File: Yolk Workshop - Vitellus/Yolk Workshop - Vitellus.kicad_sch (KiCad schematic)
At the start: 3 parts

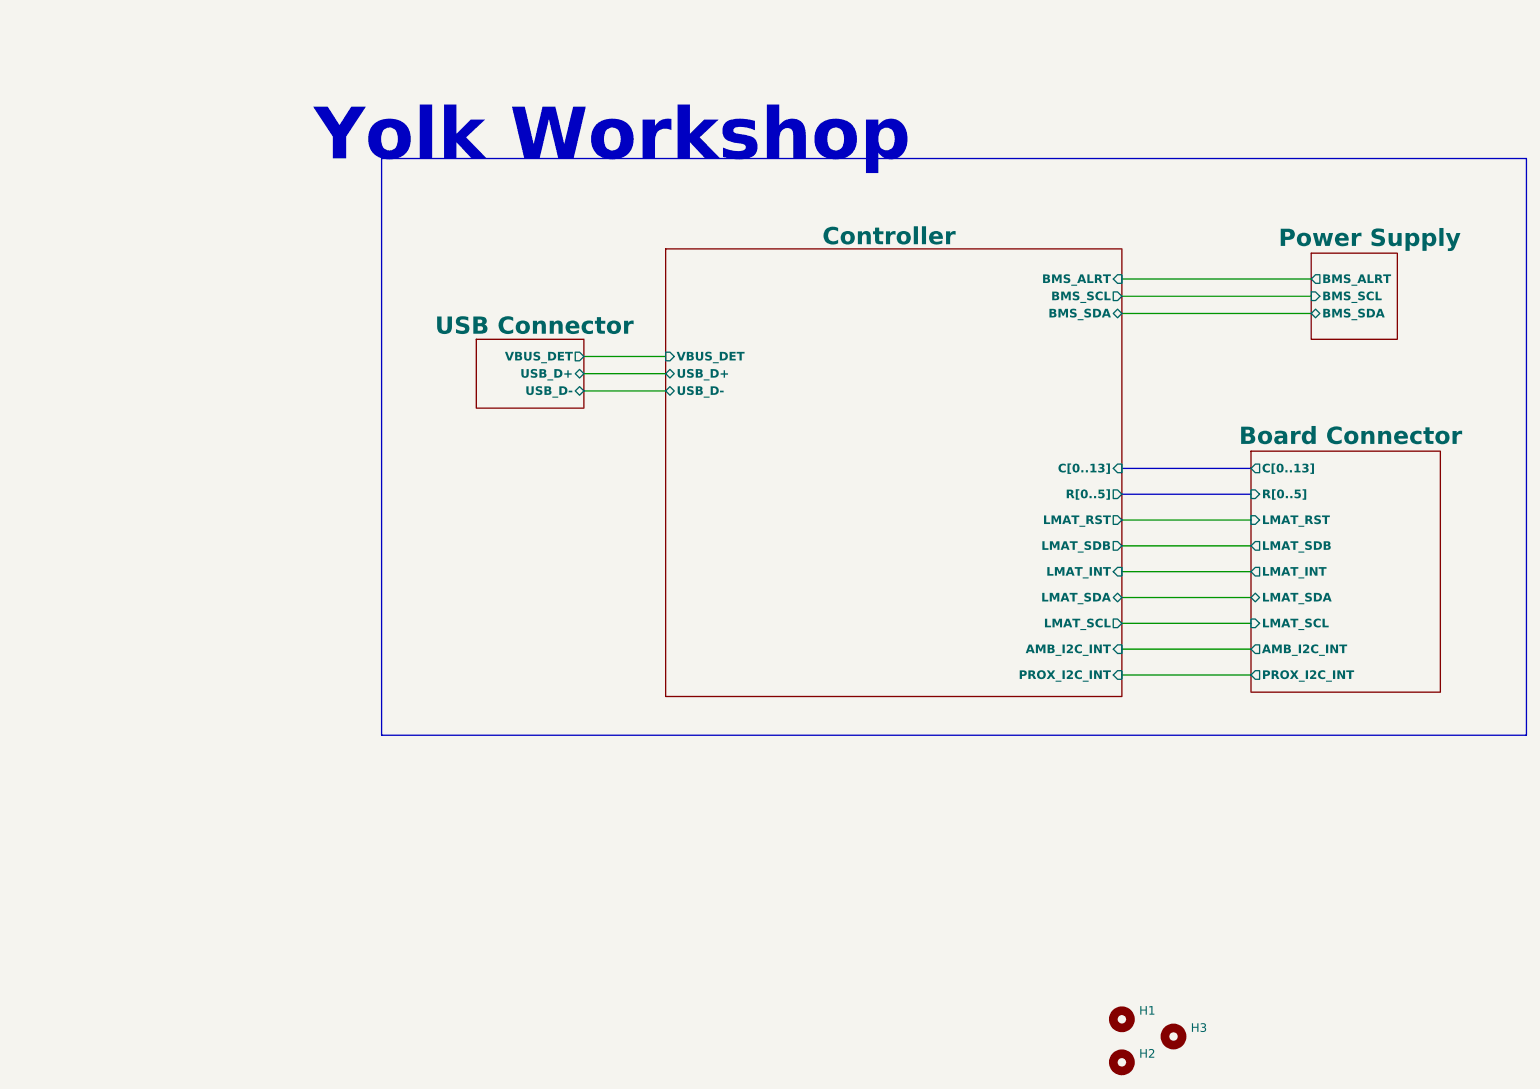
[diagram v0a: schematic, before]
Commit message: updates to HIP and Controller design
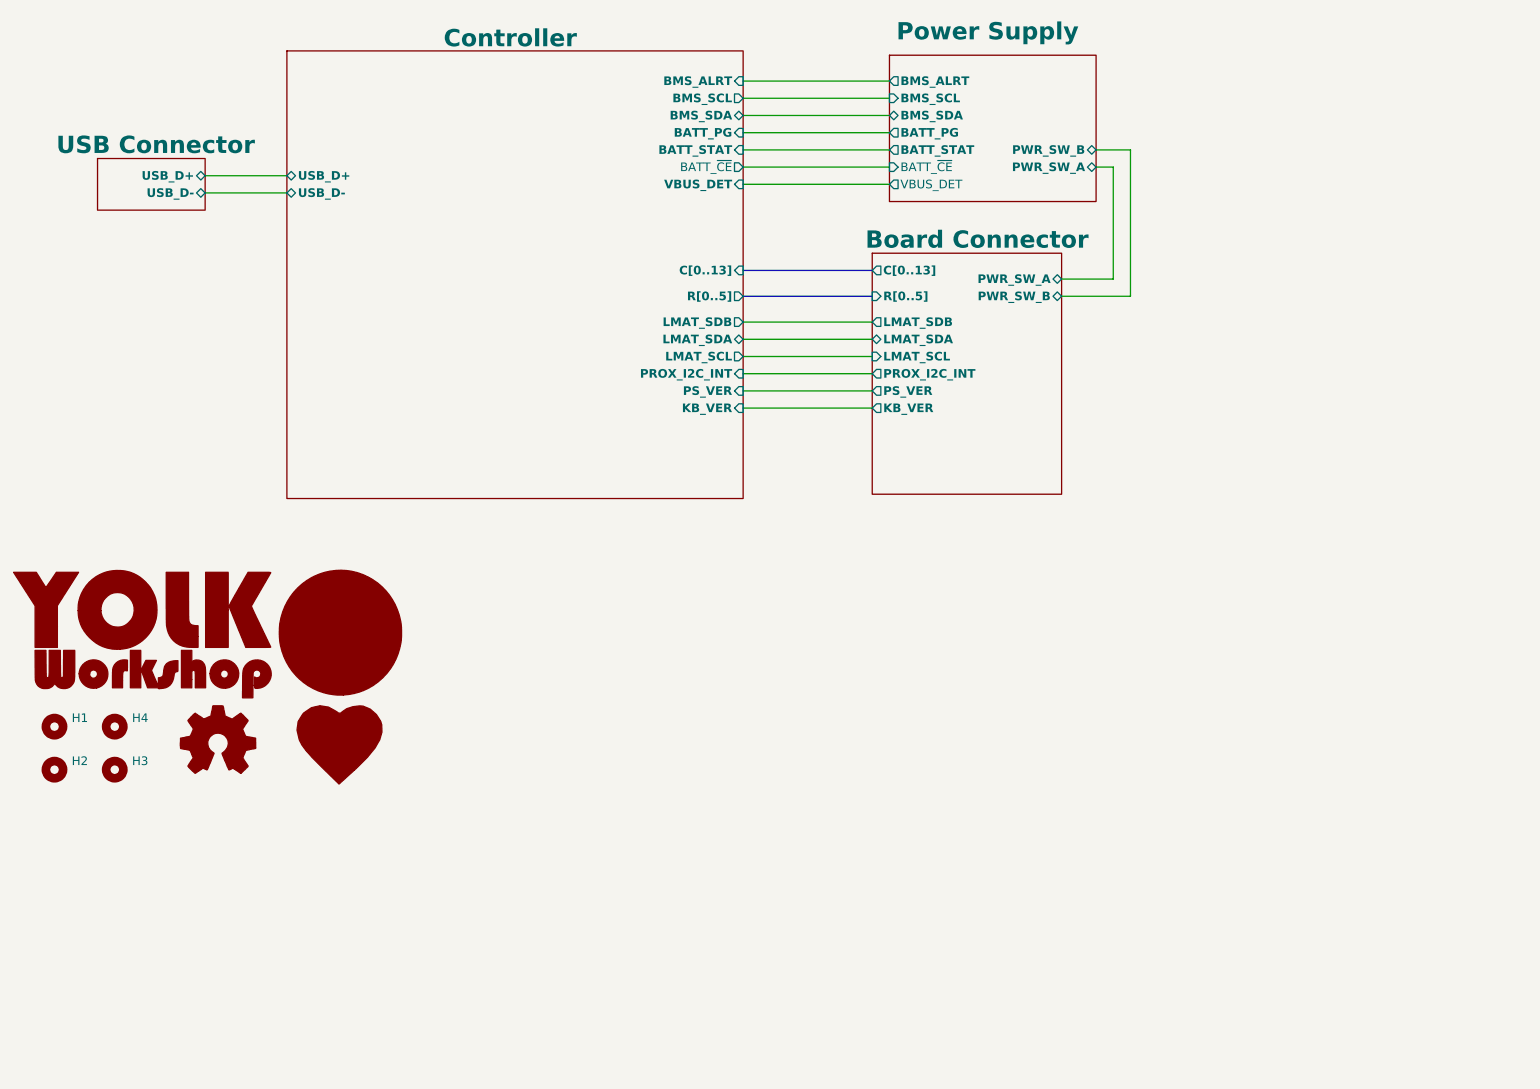
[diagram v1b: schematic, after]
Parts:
- added H4: MountingHole, MountingHole:MountingHole_2.2mm_M2_DIN965_Pad, symbol Mechanical:MountingHole
- H1, H2, H3: footprint MountingHole:MountingHole_2.2mm_M2 -> MountingHole:MountingHole_2.2mm_M2_DIN965_Pad
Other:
- sheet Board Connector ports: added KB_VER, PS_VER, PWR_SW_A, PWR_SW_B; removed AMB_I2C_INT, LMAT_INT, LMAT_RST
- sheet Controller ports: added BATT_PG, BATT_STAT, BATT_~{CE}, KB_VER, PS_VER; removed AMB_I2C_INT, LMAT_INT, LMAT_RST
- sheet Power Supply ports: added BATT_PG, BATT_STAT, BATT_~{CE}, PWR_SW_A, PWR_SW_B, VBUS_DET; removed none
- sheet USB Connector ports: added none; removed VBUS_DET
- note removed: "Yolk Workshop"
- moved on the sheet: H1, H2, H3
